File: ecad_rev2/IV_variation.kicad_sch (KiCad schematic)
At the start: 33 parts, among them U2 LM6144xIx

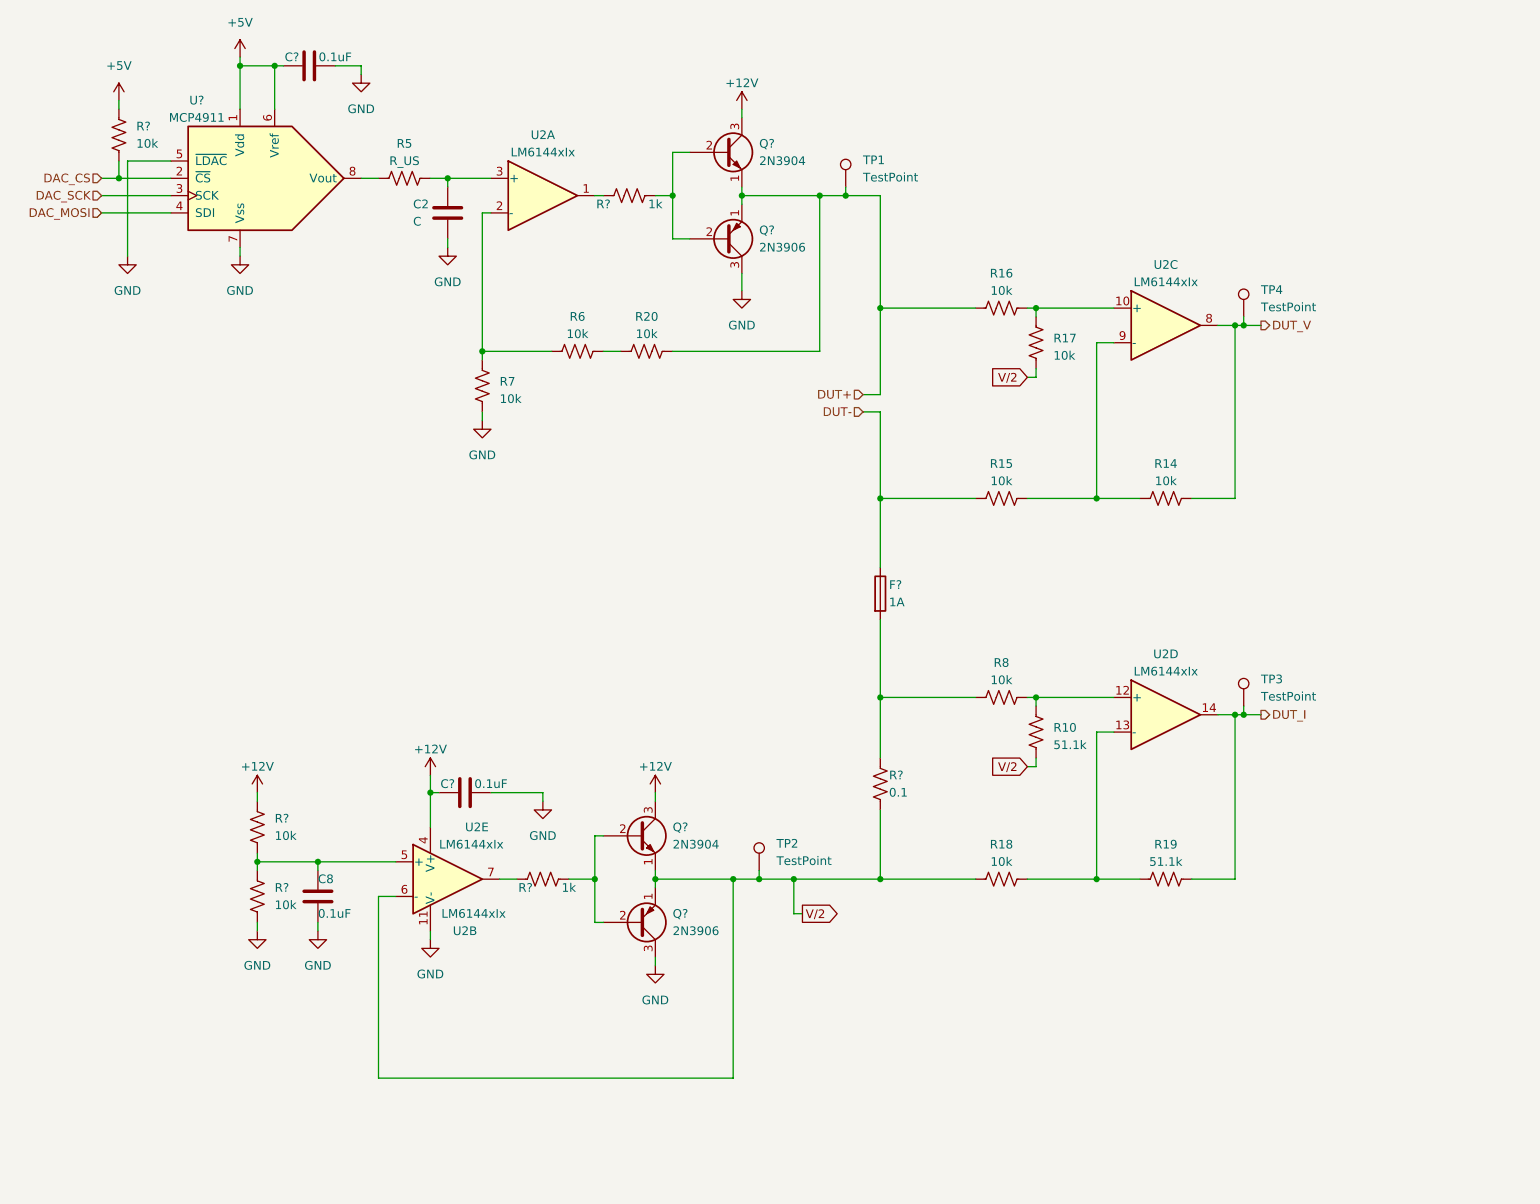
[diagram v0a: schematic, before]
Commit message: schematic work
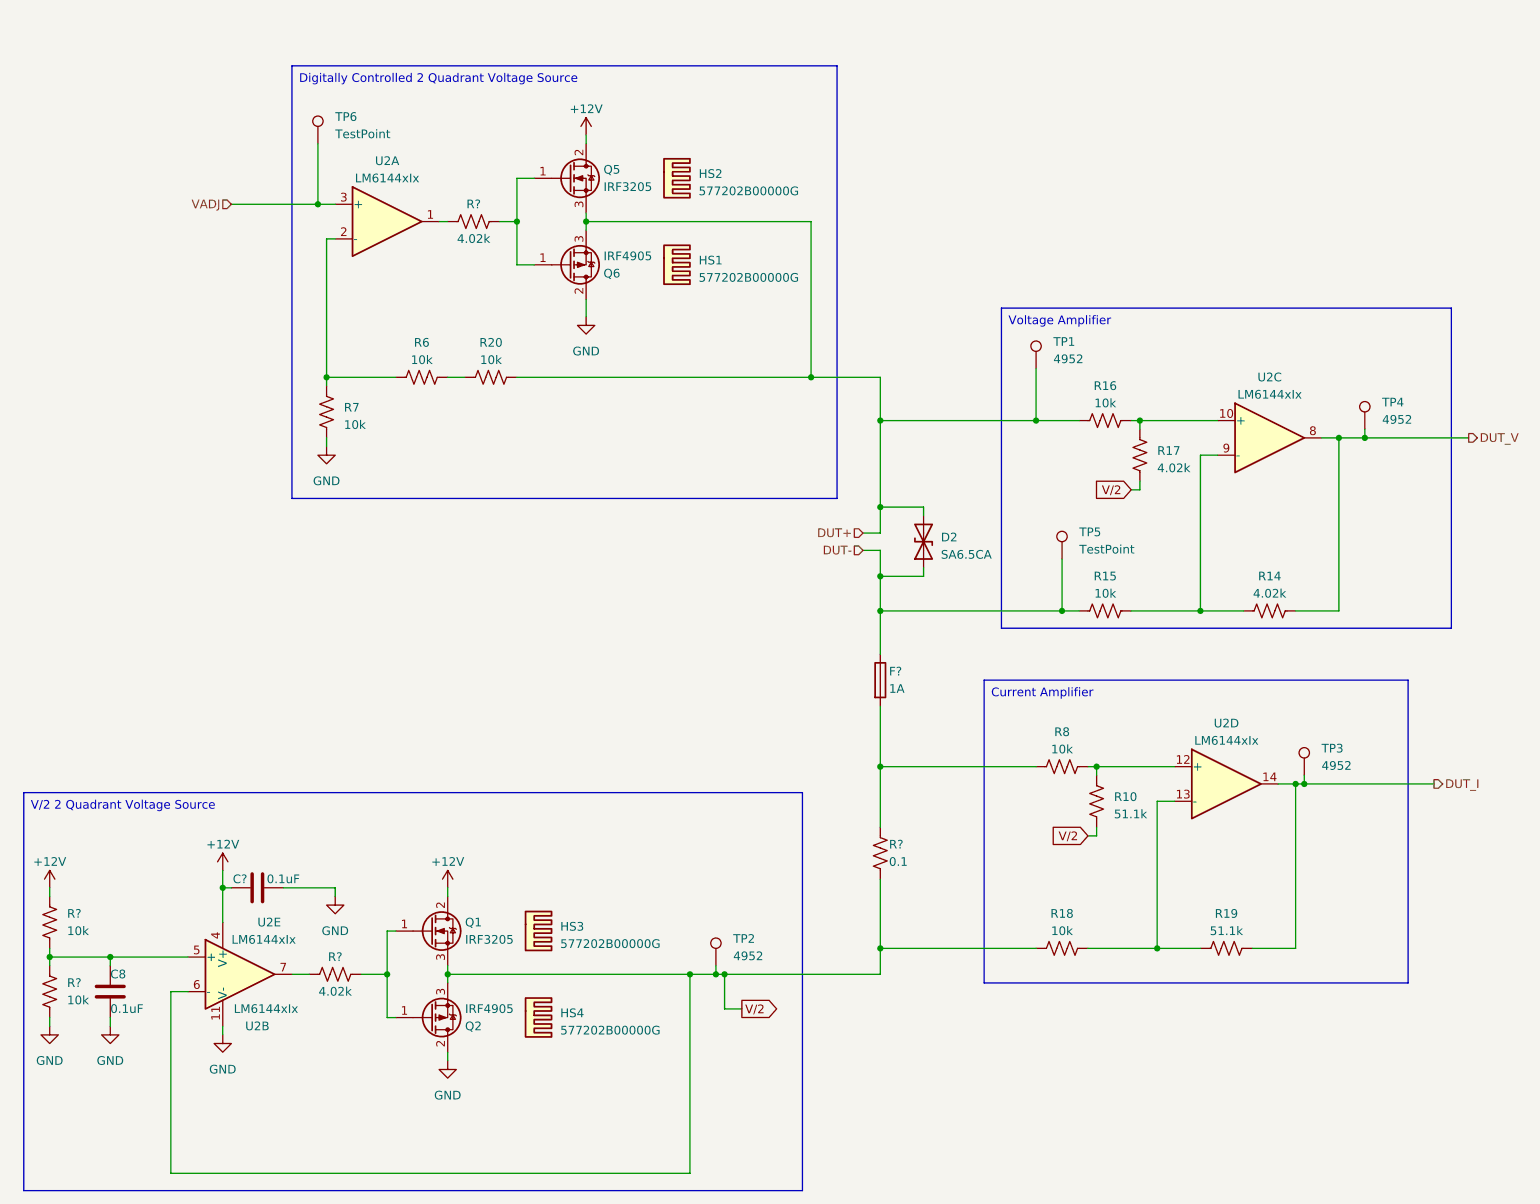
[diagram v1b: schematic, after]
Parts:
- removed C2: C, symbol Device:C
- removed C?: 0.1uF, symbol Device:C
- removed Q? (x2): 2N3904, Package_TO_SOT_THT:TO-92_Inline, symbol Transistor_BJT:2N3904
- removed Q? (x2): 2N3906, Package_TO_SOT_THT:TO-92_Inline, symbol Transistor_BJT:2N3906
- removed R5: R_US, symbol Device:R_US
- removed R?: 10k, symbol Device:R_US
- removed U?: MCP4911, symbol Analog_DAC:MCP4911
- added D2: SA6.5CA, symbol Device:D_TVS
- added HS1, HS2, HS3, HS4: 577202B00000G, symbol Mechanical:Heatsink
- added Q1, Q5: IRF3205, Package_TO_SOT_THT:TO-220-3_Vertical, symbol Transistor_FET:IRF3205
- added Q2, Q6: IRF4905, Package_TO_SOT_THT:TO-220-3_Vertical, symbol Transistor_FET:IRF4905
- added TP5, TP6: TestPoint, symbol Connector:TestPoint
- C8, C?: footprint (none) -> Capacitor_THT:C_Disc_D6.0mm_W2.5mm_P5.00mm
- R10, R15, R16, R18, R19, R20, R6, R7, R8, R? (x3): footprint (none) -> Resistor_THT:R_Axial_DIN0207_L6.3mm_D2.5mm_P7.62mm_Horizontal
- R14, R17: value 10k -> 4.02k; footprint (none) -> Resistor_THT:R_Axial_DIN0207_L6.3mm_D2.5mm_P7.62mm_Horizontal
- R? (x2): value 1k -> 4.02k; footprint (none) -> Resistor_THT:R_Axial_DIN0207_L6.3mm_D2.5mm_P7.62mm_Horizontal
- TP1, TP2, TP3, TP4: value TestPoint -> 4952
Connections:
- net +12V: now also Q1.2 (D), Q5.2 (D)
- net DUT+: now also D2.2 (A2), Q5.3 (S), Q6.3 (S)
- net DUT-: now also D2.1 (A1), TP5.1
- net GND: now also Q2.2 (D), Q6.2 (D)
- net V/2: now also Q1.3 (S), Q2.3 (S)
- net VADJ: now reaches U2.3 (+)
- net VADJ: now also TP6.1
- net at R?.2: now also Q5.1 (G), Q6.1 (G)
- net at R?.2: now also Q1.1 (G), Q2.1 (G)
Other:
- moved on the sheet: C8, C?, F?, R10, R14, R15, R16, R17, R18, R19, R20, R6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
